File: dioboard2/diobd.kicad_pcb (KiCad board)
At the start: 2 copper layers, 53.3 x 15.2 mm, 9 parts, among them J1 Conn_01x03, J2 Conn_01x03, J3 Conn_01x03, J4 Conn_01x03

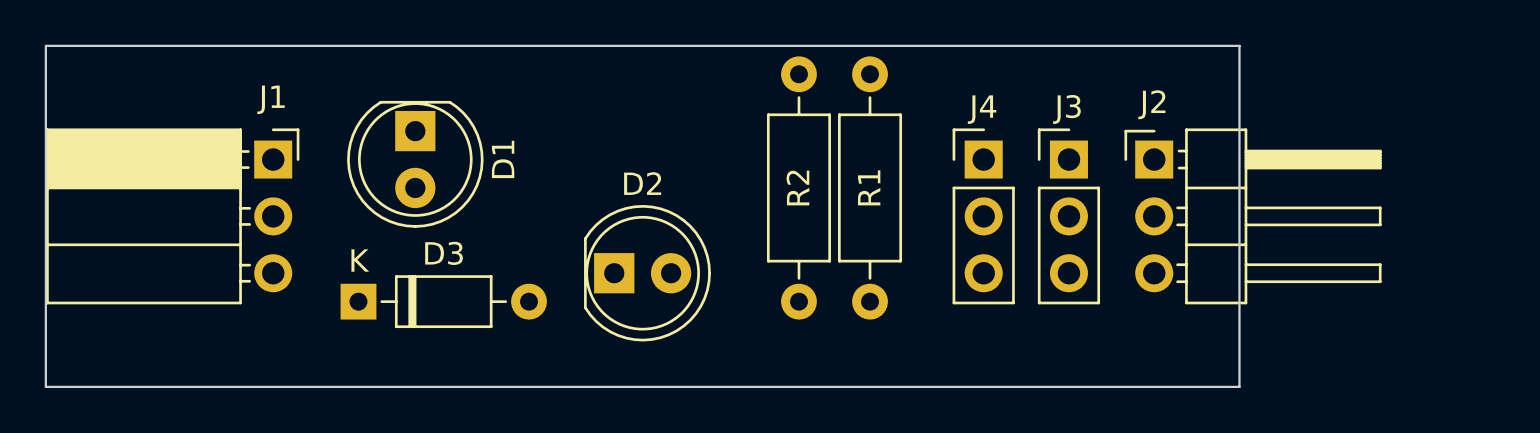
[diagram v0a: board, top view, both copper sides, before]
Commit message: Resolve Merge Error
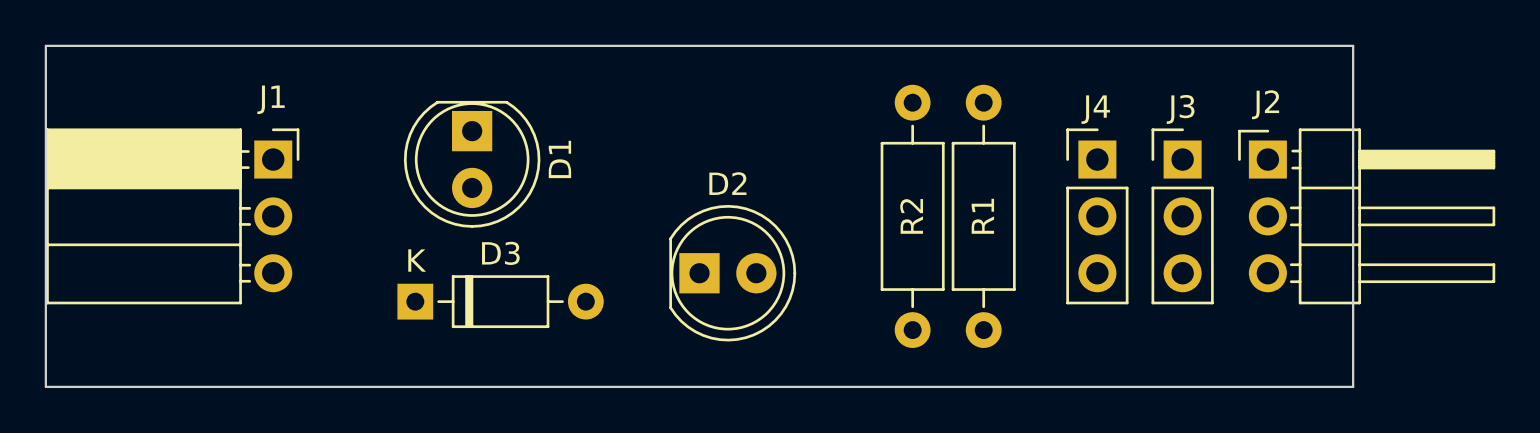
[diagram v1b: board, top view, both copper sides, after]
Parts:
- moved R2 5.24 mm to (132.7, 90.2)
- moved R1 5.24 mm to (135.9, 90.2)
- moved J2 5.08 mm to (148.6, 92.7)
- moved J3 5.08 mm to (144.8, 92.7)
- moved J4 5.08 mm to (141.0, 92.7)
- moved D2 3.81 mm to (123.2, 97.8)
- moved D1 2.54 mm to (113.0, 91.4)
- moved D3 2.54 mm to (110.5, 99.1)
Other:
- board size 53.3 x 15.2 mm -> 58.4 x 15.2 mm
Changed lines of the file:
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@@
-(kicad_pcb (version 20171130) (host pcbnew "(5.0.1)-3")
+(kicad_pcb (version 20171130) (host pcbnew 5.0.1-33cea8e~68~ubuntu16.04.1)
   (general
     (thickness 1.5748)
@@
     (aux_axis_origin 0 0)
     (grid_origin 93.98 102.87)
-    (visible_elements 7FFFFFFF)
+    (visible_elements FFFFFF7F)
     (pcbplotparams
       (layerselection 0x010fc_ffffffff)
@@
   )
   (module LED_THT:LED_D5.0mm (layer F.Cu)
-    (at 110.49 91.44 270)
+    (at 113.03 91.44 270)
     (descr "LED, diameter 5.0mm, 2 pins, http://cdn-reichelt.de/documents/datenblatt/A500/LL-504BC2E-009.pdf")
     (tags "LED diameter 5.0mm 2 pins")
@@
   )
   (module LED_THT:LED_D5.0mm (layer F.Cu)
-    (at 119.38 97.79)
+    (at 123.19 97.79)
     (descr "LED, diameter 5.0mm, 2 pins, http://cdn-reichelt.de/documents/datenblatt/A500/LL-504BC2E-009.pdf")
     (tags "LED diameter 5.0mm 2 pins")
@@
   )
   (module Diode_THT:D_DO-35_SOD27_P7.62mm_Horizontal (layer F.Cu)
-    (at 107.95 99.06)
+    (at 110.49 99.06)
     (descr "Diode, DO-35_SOD27 series, Axial, Horizontal, pin pitch=7.62mm, , length*diameter=4*2mm^2, , http://www.diodes.com/_files/packages/DO-35.pdf")
     (tags "Diode DO-35_SOD27 series Axial Horizontal pin pitch 7.62mm  length 4mm diameter 2mm")
@@
   )
   (module Connector_PinHeader_2.54mm:PinHeader_1x03_P2.54mm_Horizontal (layer F.Cu)
-    (at 143.51 92.71)
+    (at 148.59 92.71)
     (descr "Through hole angled pin header, 1x03, 2.54mm pitch, 6mm pin length, single row")
     (tags "Through hole angled pin header THT 1x03 2.54mm single row")
@@
   )
   (module Connector_PinHeader_2.54mm:PinHeader_1x03_P2.54mm_Vertical (layer F.Cu)
-    (at 139.7 92.71)
+    (at 144.78 92.71)
     (descr "Through hole straight pin header, 1x03, 2.54mm pitch, single row")
     (tags "Through hole pin header THT 1x03 2.54mm single row")
@@
   )
   (module Connector_PinHeader_2.54mm:PinHeader_1x03_P2.54mm_Vertical (layer F.Cu)
-    (at 135.89 92.71)
+    (at 140.97 92.71)
     (descr "Through hole straight pin header, 1x03, 2.54mm pitch, single row")
     (tags "Through hole pin header THT 1x03 2.54mm single row")
@@
   )
   (module Resistor_THT:R_Axial_DIN0207_L6.3mm_D2.5mm_P10.16mm_Horizontal (layer F.Cu)
-    (at 130.81 88.9 270)
+    (at 135.89 90.17 270)
     (descr "Resistor, Axial_DIN0207 series, Axial, Horizontal, pin pitch=10.16mm, 0.25W = 1/4W, length*diameter=6.3*2.5mm^2, http://cdn-reichelt.de/documents/datenblatt/B400/1_4W%23YAG.pdf")
     (tags "Resistor Axial_DIN0207 series Axial Horizontal pin pitch 10.16mm 0.25W = 1/4W length 6.3mm diameter 2.5mm")
@@
   )
   (module Resistor_THT:R_Axial_DIN0207_L6.3mm_D2.5mm_P10.16mm_Horizontal (layer F.Cu)
-    (at 127.635 88.9 270)
+    (at 132.715 90.17 270)
     (descr "Resistor, Axial_DIN0207 series, Axial, Horizontal, pin pitch=10.16mm, 0.25W = 1/4W, length*diameter=6.3*2.5mm^2, http://cdn-reichelt.de/documents/datenblatt/B400/1_4W%23YAG.pdf")
     (tags "Resistor Axial_DIN0207 series Axial Horizontal pin pitch 10.16mm 0.25W = 1/4W length 6.3mm diameter 2.5mm")
@@
   )
   (gr_line (start 93.98 87.63) (end 93.98 102.87) (layer Edge.Cuts) (width 0.1))
-  (gr_line (start 147.32 87.63) (end 93.98 87.63) (layer Edge.Cuts) (width 0.1))
-  (gr_line (start 147.32 102.87) (end 147.32 87.63) (layer Edge.Cuts) (width 0.1))
-  (gr_line (start 93.98 102.87) (end 147.32 102.87) (layer Edge.Cuts) (width 0.1))
+  (gr_line (start 152.4 87.63) (end 93.98 87.63) (layer Edge.Cuts) (width 0.1))
+  (gr_line (start 152.4 102.87) (end 152.4 87.63) (layer Edge.Cuts) (width 0.1))
+  (gr_line (start 93.98 102.87) (end 152.4 102.87) (layer Edge.Cuts) (width 0.1))
 )
